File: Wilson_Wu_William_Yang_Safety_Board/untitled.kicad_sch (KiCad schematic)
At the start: 44 parts, among them J3 430450200, J5 430450200, J6 XT60-M, J7 XT60-M, Q1 IRLML6344TRPBF, Q2 IRLML6344TRPBF, Q3 NTBLS0D8N08XTXG, Q4 NTBLS0D8N08XTXG, U10 LTC4364HS, U16 J115F11AH12VDCS61.5U, U5 J115F11AH12VDCS61.5U, U6 J115F11AH12VDCS61.5U

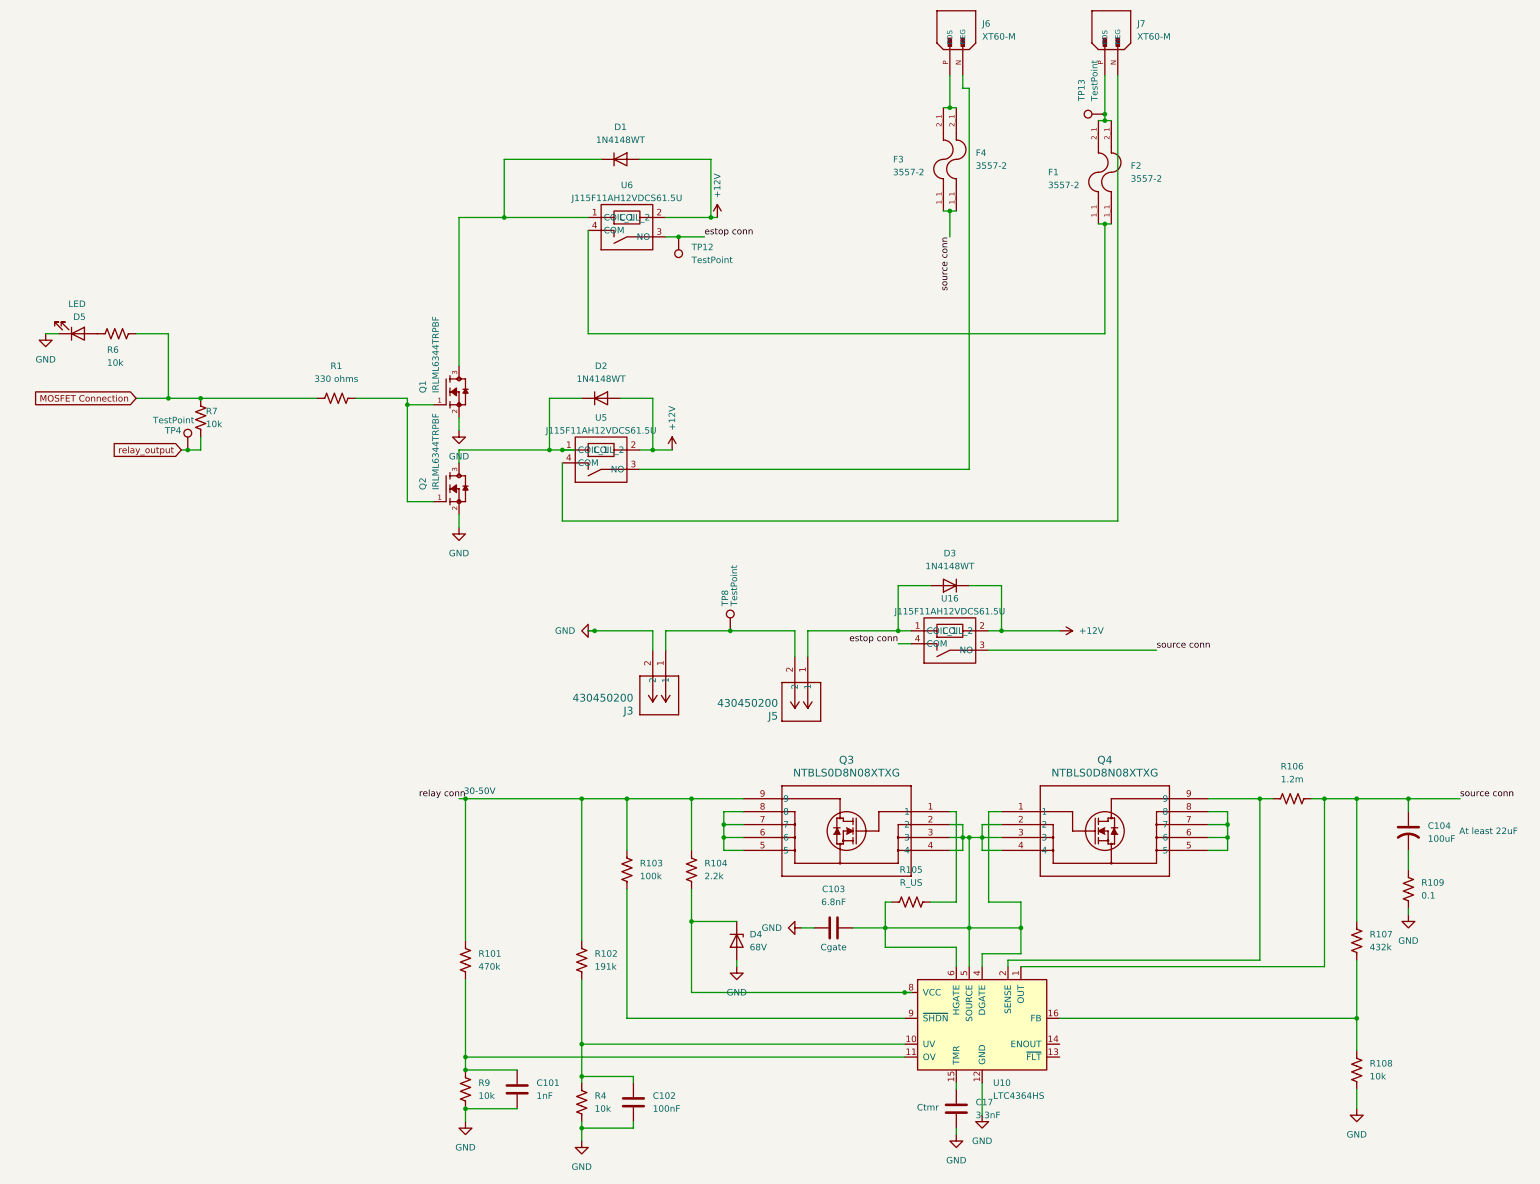
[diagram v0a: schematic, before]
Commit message: sch changes
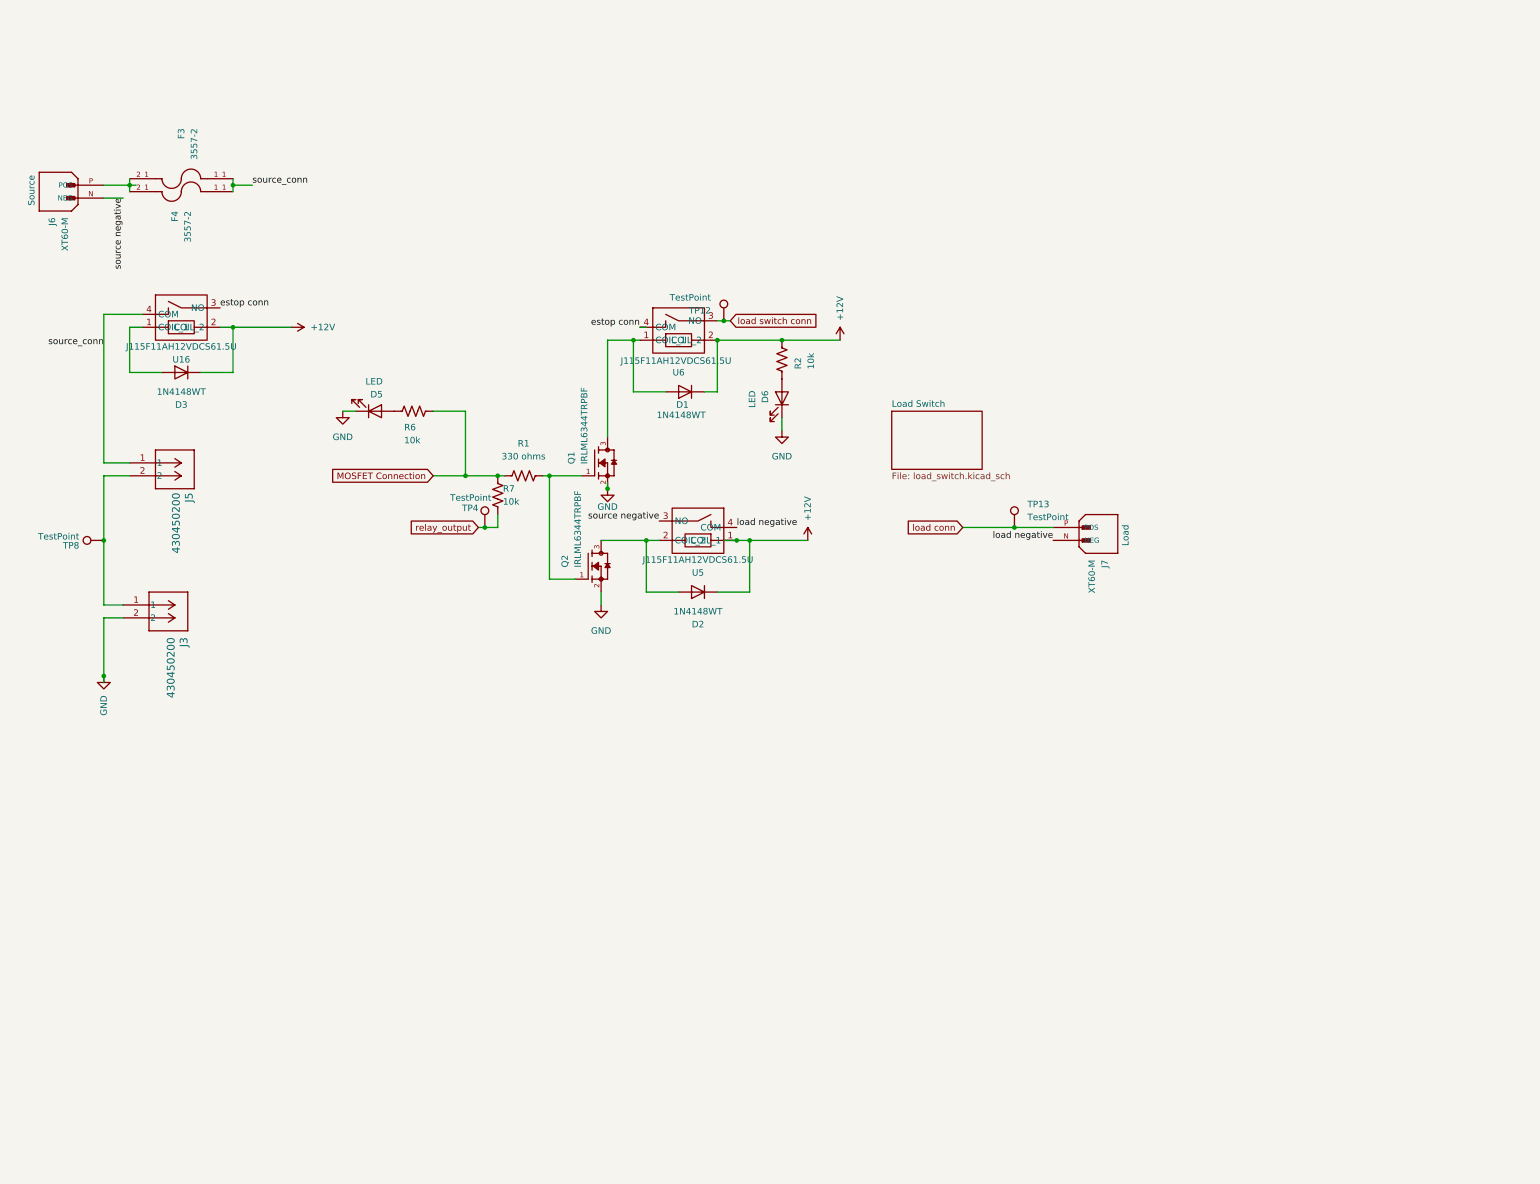
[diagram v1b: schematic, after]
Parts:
- removed C101: 1nF, SMV_Passives:CAPC17595_87N_KEM, symbol Device:C
- removed C102: 100nF, SMV_Passives:CAPC17595_87N_KEM, symbol Device:C
- removed C103: 6.8nF, SMV_Passives:CAPC17595_87N_KEM, symbol Device:C
- removed C104: 100uF, SMV_Passives:CAPC17595_87N_KEM, symbol Device:C_US
- removed C17: 3.3nF, SMV_Passives:CAPC17595_87N_KEM, symbol Device:C
- removed D4: 68V, symbol Device:D_Zener
- removed F1, F2: 3557-2, SMV_Connectors:FUSE_3557-2, symbol SMV_Custom:3555-2
- removed Q3, Q4: NTBLS0D8N08XTXG, H-PSOF8L_100CU_ONS_OSI, symbol SMV_beefy_FET:NTBLS0D8N08XTXG
- removed R101: 470k, SMV_Passives:0603_resistors, symbol Device:R_US
- removed R102: 191k, SMV_Passives:0603_resistors, symbol Device:R_US
- removed R103: 100k, SMV_Passives:0603_resistors, symbol Device:R_US
- removed R104: 2.2k, SMV_Passives:0603_resistors, symbol Device:R_US
- removed R105: R_US, SMV_Passives:0603_resistors, symbol Device:R_US
- removed R106: 1.2m, SMV_Passives:0603_resistors, symbol Device:R_US
- removed R107: 432k, SMV_Passives:0603_resistors, symbol Device:R_US
- removed R108, R4, R9: 10k, SMV_Passives:0603_resistors, symbol Device:R_US
- removed R109: 0.1, SMV_Passives:0603_resistors, symbol Device:R_US
- removed U10: LTC4364HS, Package_SO:SOIC-16_3.9x9.9mm_P1.27mm, symbol Power_Management:LTC4364HS
- added D6: LED, LED_SMD:LED_Foshan-NTD3528_3.5x2.8mm, symbol Device:LED
- added R2: 10k, Resistor_SMD:R_0805_2012Metric, symbol Device:R_US
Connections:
- net +12V: now also D1.1 (K), D2.1 (K), U5.1 (COIL_1), R2.2; no longer D1.2 (A), D2.2 (A), U5.2 (COIL_2)
- net GND: now also D6.1 (K)
- net estop conn: now also U16.3 (NO), U6.4 (COM); no longer TP12.1, U16.4 (COM), U6.3 (NO)
- net load negative: now reaches J7.N (NEG), U5.4 (COM)
- net load conn: now reaches J7.P (POS), TP13.1
- net at Q1.3, U6.1 (COIL_1): now also D1.2 (A); no longer D1.1 (K)
- net at D3.2 (A), U16.1 (COIL_1): no longer J5.1
- net source negative: now reaches J6.N (NEG), U5.3 (NO)
- net source conn renamed source_conn
- net source_conn: now also J5.1, U16.4 (COM); no longer U16.3 (NO)
- new net: D6.2 (A), R2.1
- new net: D2.2 (A), Q2.3, U5.2 (COIL_2)
- new net load switch conn: TP12.1, U6.3 (NO)
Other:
- added sheet Load Switch (load_switch.kicad_sch)
- note added: "Load"
- note added: "Source"
- note removed: "30-50V"
- note removed: "At least 22uF"
- note removed: "Cgate"
- note removed: "Ctmr"
- moved on the sheet: D1, D2, D3, D5, F3, F4, J3, J5, J6, J7, Q1, Q2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
